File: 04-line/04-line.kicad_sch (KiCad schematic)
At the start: 71 parts, among them J1 Conn_01x10, J2 Conn_01x10, J3 Conn_01x08

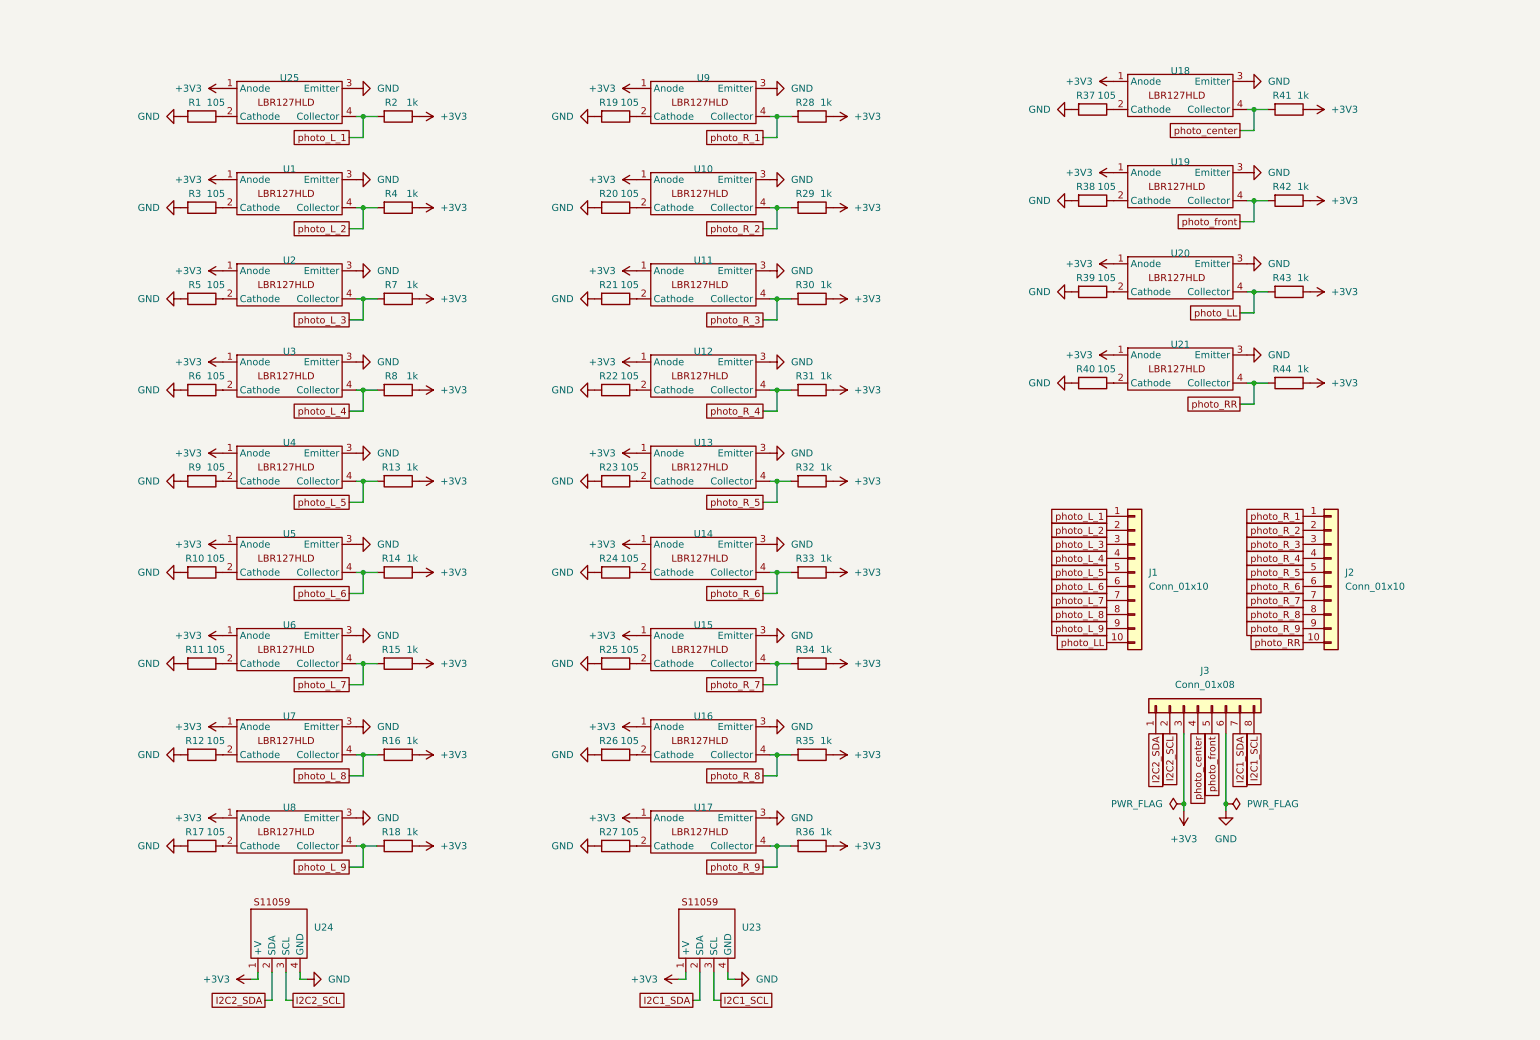
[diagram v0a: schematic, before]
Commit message: がんばる
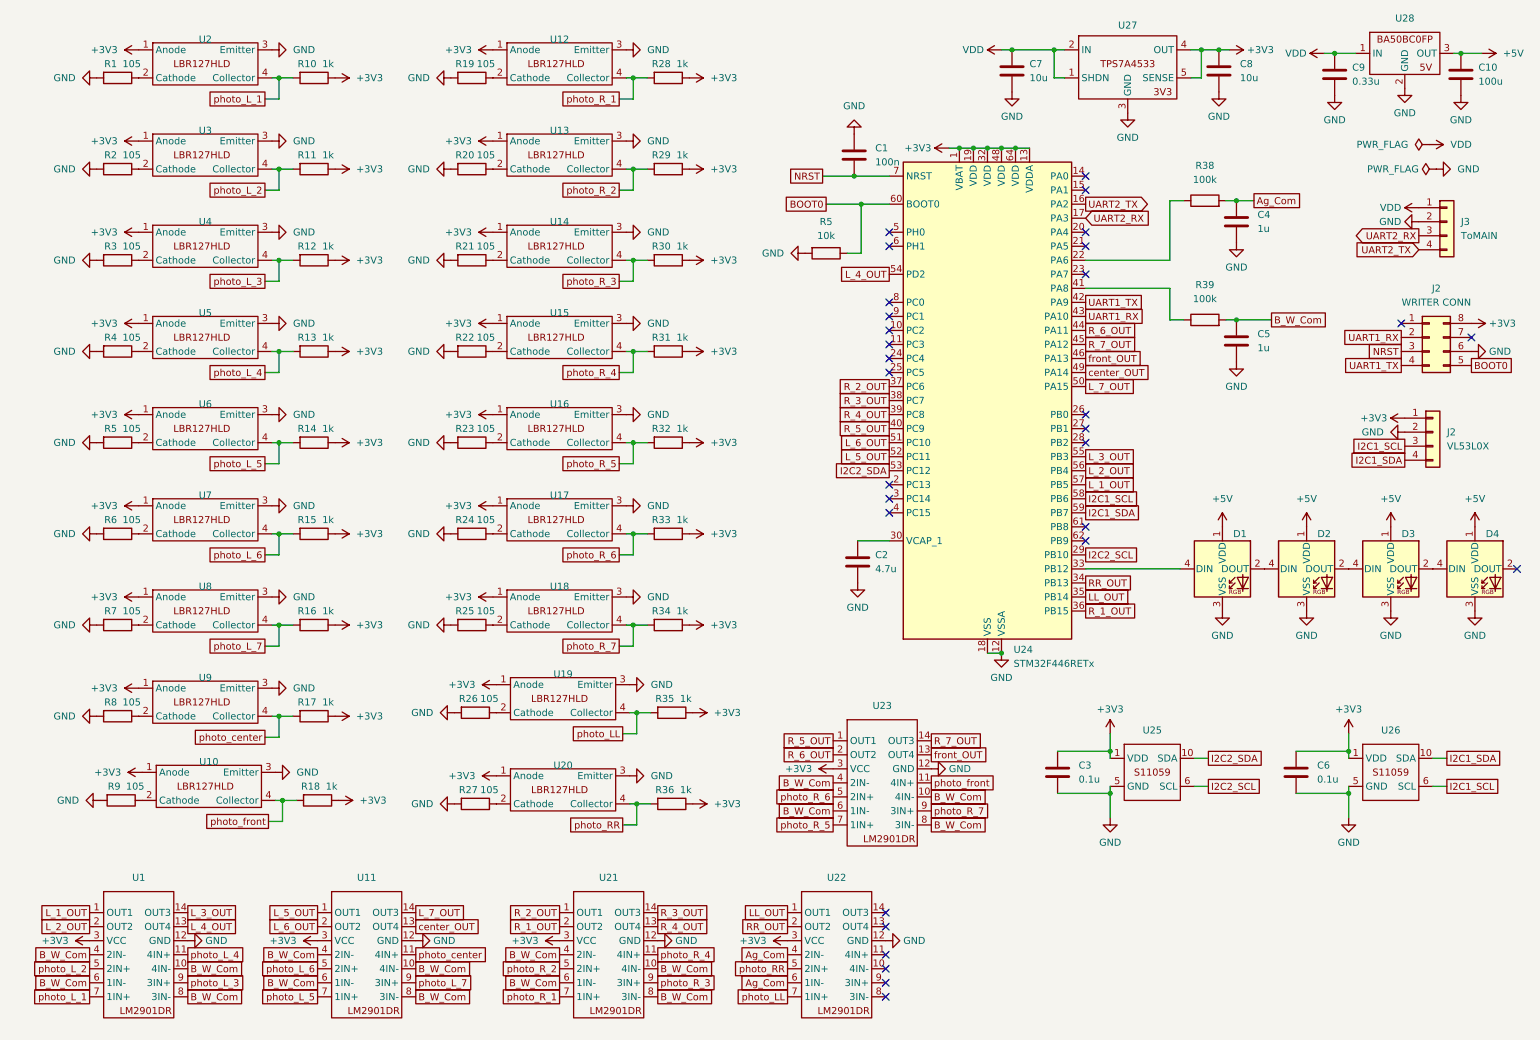
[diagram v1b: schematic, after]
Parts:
- removed J1, J2: Conn_01x10, Connector_PinHeader_2.54mm:PinHeader_1x10_P2.54mm_Vertical, symbol Connector_Generic:Conn_01x10
- removed J3: Conn_01x08, Connector_PinHeader_2.54mm:PinHeader_1x08_P2.54mm_Vertical, symbol Connector_Generic:Conn_01x08
- removed R12, R17, R26, R27: 105, symbol Device:R
- removed R16, R18, R35, R36: 1k, symbol Device:R
- removed U16, U17, U7, U8: ~, symbol akiduki:LBR127HLD
- removed U23, U24: ~, S11059:S11059, symbol S11059:S11059
- added C1: 100n, symbol Device:C
- added C10: 100u, symbol Device:C
- added C2: 4.7u, symbol Device:C
- added C3, C6: 0.1u, symbol Device:C
- added C4, C5: 1u, symbol Device:C
- added C7, C8: 10u, symbol Device:C
- added C9: 0.33u, symbol Device:C
- added D1, D2, D3, D4: WS2812B, LED_SMD:LED_WS2812B_PLCC4_5.0x5.0mm_P3.2mm, symbol LED:WS2812B
- added J2: VL53L0X, Connector_PinHeader_2.54mm:PinHeader_1x04_P2.54mm_Vertical, symbol Connector_Generic:Conn_01x04
- added J2: WRITER CONN, Connector_PinHeader_2.54mm:PinHeader_2x04_P2.54mm_Vertical, symbol Connector_Generic:Conn_02x04_Counter_Clockwise
- added J3: ToMAIN, Connector_JST:JST_XH_B4B-XH-A_1x04_P2.50mm_Vertical, symbol Connector_Generic:Conn_01x04
- added R38, R39: 100k, symbol Device:R
- added R5: 10k, Resistor_SMD:R_0805_2012Metric, symbol Device:R
- added U1, U11, U21, U22, U23: ~, Package_SO:SOIC-14_3.9x8.7mm_P1.27mm, symbol JLCPCB_items:LM2901DR
- added U24: STM32F446RETx, Package_QFP:LQFP-64_10x10mm_P0.5mm, symbol MCU_ST_STM32F4:STM32F446RETx
- added U25, U26: ~, Akiduki:S11059, symbol akiduki:S11059
- added U27: ~, Package_TO_SOT_SMD:SOT-223-6, symbol JLCPCB_items:TPS7A4533DCQR
- added U28: ~, Package_TO_SOT_SMD:TO-252-3_TabPin2, symbol JLCPCB_items:BA50BC0FP
- R1, R19, R20, R21, R22, R23, R24, R25: footprint (none) -> Resistor_SMD:R_0603_1608Metric; LCSC (none) -> C128061
- R10: renamed from R2; footprint (none) -> Resistor_SMD:R_1206_3216Metric; LCSC (none) -> C138242
- R11: renamed from R4; footprint (none) -> Resistor_SMD:R_1206_3216Metric; LCSC (none) -> C138242
- R12: renamed from R7; footprint (none) -> Resistor_SMD:R_1206_3216Metric; LCSC (none) -> C138242
- R13: renamed from R8; footprint (none) -> Resistor_SMD:R_1206_3216Metric; LCSC (none) -> C138242
- R14: renamed from R13; footprint (none) -> Resistor_SMD:R_1206_3216Metric; LCSC (none) -> C138242
- R15: renamed from R14; footprint (none) -> Resistor_SMD:R_1206_3216Metric; LCSC (none) -> C138242
- R16: renamed from R15; footprint (none) -> Resistor_SMD:R_1206_3216Metric; LCSC (none) -> C138242
- R17: renamed from R41; footprint (none) -> Resistor_SMD:R_1206_3216Metric; LCSC (none) -> C138242
- R18: renamed from R42; footprint (none) -> Resistor_SMD:R_1206_3216Metric; LCSC (none) -> C138242
- R2: renamed from R3; footprint (none) -> Resistor_SMD:R_0603_1608Metric; LCSC (none) -> C128061
- R26: renamed from R39; footprint (none) -> Resistor_SMD:R_0603_1608Metric; LCSC (none) -> C128061
- R27: renamed from R40; footprint (none) -> Resistor_SMD:R_0603_1608Metric; LCSC (none) -> C128061
- R28, R29, R30, R31, R32, R33, R34: footprint (none) -> Resistor_SMD:R_1206_3216Metric; LCSC (none) -> C138242
- R3: renamed from R5; footprint (none) -> Resistor_SMD:R_0603_1608Metric; LCSC (none) -> C128061
- R35: renamed from R43; footprint (none) -> Resistor_SMD:R_1206_3216Metric; LCSC (none) -> C138242
- R36: renamed from R44; footprint (none) -> Resistor_SMD:R_1206_3216Metric; LCSC (none) -> C138242
- R4: renamed from R6; footprint (none) -> Resistor_SMD:R_0603_1608Metric; LCSC (none) -> C128061
- R5: renamed from R9; footprint (none) -> Resistor_SMD:R_0603_1608Metric; LCSC (none) -> C128061
- R6: renamed from R10; footprint (none) -> Resistor_SMD:R_0603_1608Metric; LCSC (none) -> C128061
- R7: renamed from R11; footprint (none) -> Resistor_SMD:R_0603_1608Metric; LCSC (none) -> C128061
- R8: renamed from R37; footprint (none) -> Resistor_SMD:R_0603_1608Metric; LCSC (none) -> C128061
- R9: renamed from R38; footprint (none) -> Resistor_SMD:R_0603_1608Metric; LCSC (none) -> C128061
- U10: renamed from U19; footprint (none) -> Akiduki:LBR127HLD
- U12: renamed from U9; footprint (none) -> Akiduki:LBR127HLD
- U13: renamed from U10; footprint (none) -> Akiduki:LBR127HLD
- U14: renamed from U11; footprint (none) -> Akiduki:LBR127HLD
- U15: renamed from U12; footprint (none) -> Akiduki:LBR127HLD
- U16: renamed from U13; footprint (none) -> Akiduki:LBR127HLD
- U17: renamed from U14; footprint (none) -> Akiduki:LBR127HLD
- U18: renamed from U15; footprint (none) -> Akiduki:LBR127HLD
- U19: renamed from U20; footprint (none) -> Akiduki:LBR127HLD
- U2: renamed from U25; footprint (none) -> Akiduki:LBR127HLD
- U20: renamed from U21; footprint (none) -> Akiduki:LBR127HLD
- U3: renamed from U1; footprint (none) -> Akiduki:LBR127HLD
- U4: renamed from U2; footprint (none) -> Akiduki:LBR127HLD
- U5: renamed from U3; footprint (none) -> Akiduki:LBR127HLD
- U6: renamed from U4; footprint (none) -> Akiduki:LBR127HLD
- U7: renamed from U5; footprint (none) -> Akiduki:LBR127HLD
- U8: renamed from U6; footprint (none) -> Akiduki:LBR127HLD
- U9: renamed from U18; footprint (none) -> Akiduki:LBR127HLD
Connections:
- net +3V3: now also C3.1, C6.1, C8.1, J2.1 (Pin_1), J2.8 (Pin_8), U1.3 (VCC), U11.3 (VCC), U21.3 (VCC), U22.3 (VCC), U23.3 (VCC), U24.1 (VBAT), U24.13 (VDDA), U24.19 (VDD), U24.32 (VDD), U24.48 (VDD), U24.64 (VDD), U25.1 (VDD), U26.1 (VDD), U27.4 (OUT), U27.5 (SENSE)
- net GND: now also C1.1, C10.2, C2.2, C3.2, C4.2, C5.2, C6.2, C7.2, C8.2, C9.2, D1.3 (VSS), D2.3 (VSS), D3.3 (VSS), D4.3 (VSS), J2.2 (Pin_2), J2.6 (Pin_6), J3.2 (Pin_2), R5.2, U1.12 (GND), U11.12 (GND), U21.12 (GND), U22.12 (GND), U23.12 (GND), U24.12 (VSSA), U24.18 (VSS), U24.31 (VSS), U24.47 (VSS), U24.63 (VSS), U25.5 (GND), U26.5 (GND), U27.3 (GND), U27.6 (GND), U28.2 (GND)
- net I2C1_SCL: now also J2.3 (Pin_3), U24.58 (PB6), U26.6 (SCL)
- net I2C1_SDA: now also J2.4 (Pin_4), U24.59 (PB7), U26.10 (SDA)
- net I2C2_SCL: now also U24.29 (PB10), U25.6 (SCL)
- net I2C2_SDA: now also U24.53 (PC12), U25.10 (SDA)
- net photo_LL: now also U22.7 (1IN+)
- net photo_L_1: now also U1.7 (1IN+)
- net photo_L_2: now also U1.5 (2IN+)
- net photo_L_3: now also U1.9 (3IN+)
- net photo_L_4: now also U1.11 (4IN+)
- net photo_L_5: now also U11.7 (1IN+)
- net photo_L_6: now also U11.5 (2IN+)
- net photo_L_7: now also U11.9 (3IN+)
- net photo_RR: now also U22.5 (2IN+)
- net photo_R_1: now also U21.7 (1IN+)
- net photo_R_2: now also U21.5 (2IN+)
- net photo_R_3: now also U21.9 (3IN+)
- net photo_R_4: now also U21.11 (4IN+)
- net photo_R_5: now also U23.7 (1IN+)
- net photo_R_6: now also U23.5 (2IN+)
- net photo_R_7: now also U23.9 (3IN+)
- net photo_center: now also U11.11 (4IN+)
- net photo_front: now also U23.11 (4IN+)
- new net: D2.2 (DOUT), D3.4 (DIN)
- new net: D1.2 (DOUT), D2.4 (DIN)
- new net: D1.4 (DIN), U24.33 (PB12)
- new net: R39.1, U24.41 (PA8)
- new net: R38.1, U24.22 (PA6)
- new net: C2.1, U24.30 (VCAP_1)
- new net: D3.2 (DOUT), D4.4 (DIN)
- new net +5V: C10.1, D1.1 (VDD), D2.1 (VDD), D3.1 (VDD), D4.1 (VDD), U28.3 (OUT)
- new net Ag_Com: C4.1, R38.2, U22.4 (2IN-), U22.6 (1IN-)
- new net BOOT0: J2.5 (Pin_5), R5.1, U24.60 (BOOT0)
- new net B_W_Com: C5.1, R39.2, U1.10 (4IN-), U1.4 (2IN-), U1.6 (1IN-), U1.8 (3IN-), U11.10 (4IN-), U11.4 (2IN-), U11.6 (1IN-), U11.8 (3IN-), U21.10 (4IN-), U21.4 (2IN-), U21.6 (1IN-), U21.8 (3IN-), U23.10 (4IN-), U23.4 (2IN-), U23.6 (1IN-), U23.8 (3IN-)
- new net LL_OUT: U22.1 (OUT1), U24.35 (PB14)
- new net L_1_OUT: U1.1 (OUT1), U24.57 (PB5)
- new net L_2_OUT: U1.2 (OUT2), U24.56 (PB4)
- new net L_3_OUT: U1.14 (OUT3), U24.55 (PB3)
- new net L_4_OUT: U1.13 (OUT4), U24.54 (PD2)
- new net L_5_OUT: U11.1 (OUT1), U24.52 (PC11)
- new net L_6_OUT: U11.2 (OUT2), U24.51 (PC10)
- new net L_7_OUT: U11.14 (OUT3), U24.50 (PA15)
- new net NRST: C1.2, J2.3 (Pin_3), U24.7 (NRST)
- new net RR_OUT: U22.2 (OUT2), U24.34 (PB13)
- new net R_1_OUT: U21.2 (OUT2), U24.36 (PB15)
- new net R_2_OUT: U21.1 (OUT1), U24.37 (PC6)
- new net R_3_OUT: U21.14 (OUT3), U24.38 (PC7)
- new net R_4_OUT: U21.13 (OUT4), U24.39 (PC8)
- new net R_5_OUT: U23.1 (OUT1), U24.40 (PC9)
- new net R_6_OUT: U23.2 (OUT2), U24.44 (PA11)
- new net R_7_OUT: U23.14 (OUT3), U24.45 (PA12)
- new net UART1_RX: J2.2 (Pin_2), U24.43 (PA10)
- new net UART1_TX: J2.4 (Pin_4), U24.42 (PA9)
- new net UART2_RX: J3.3 (Pin_3), U24.17 (PA3)
- new net UART2_TX: J3.4 (Pin_4), U24.16 (PA2)
- new net VDD: C7.1, C9.1, J3.1 (Pin_1), U27.1 (SHDN), U27.2 (IN), U28.1 (IN)
- new net center_OUT: U11.13 (OUT4), U24.49 (PA14)
- new net front_OUT: U23.13 (OUT4), U24.46 (PA13)
- no-connect marks 0 -> 30
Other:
- title: (none) -> 04-LINE
- moved on the sheet: R1, R10, R11, R12, R13, R14, R15, R16, R17, R18, R19, R2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

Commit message: line...
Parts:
- C1, C10, C2, C3, C4, C5, C6, C7, C8, C9: footprint (none) -> Capacitor_SMD:C_0805_2012Metric
- R38, R39: footprint (none) -> Resistor_SMD:R_0805_2012Metric
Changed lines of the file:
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@@
       (effects (font (size 1.27 1.27)) (justify left))
     )
-    (property "Footprint" "" (at 200.3552 154.305 0)
+    (property "Footprint" "Capacitor_SMD:C_0805_2012Metric" (at 200.3552 154.305 0)
       (effects (font (size 1.27 1.27)) hide)
     )
@@
       (effects (font (size 1.27 1.27)) (justify left))
     )
-    (property "Footprint" "" (at 229.5652 27.305 0)
+    (property "Footprint" "Capacitor_SMD:C_0805_2012Metric" (at 229.5652 27.305 0)
       (effects (font (size 1.27 1.27)) hide)
     )
@@
       (effects (font (size 1.27 1.27)) (justify left))
     )
-    (property "Footprint" "" (at 163.5252 42.545 0)
+    (property "Footprint" "Capacitor_SMD:C_0805_2012Metric" (at 163.5252 42.545 0)
       (effects (font (size 1.27 1.27)) hide)
     )
@@
       (effects (font (size 1.27 1.27)) (justify left))
     )
-    (property "Footprint" "" (at 192.1002 27.305 0)
+    (property "Footprint" "Capacitor_SMD:C_0805_2012Metric" (at 192.1002 27.305 0)
       (effects (font (size 1.27 1.27)) hide)
     )
@@
       (effects (font (size 1.27 1.27)) (justify left))
     )
-    (property "Footprint" "" (at 232.7402 54.61 0)
+    (property "Footprint" "Capacitor_SMD:C_0805_2012Metric" (at 232.7402 54.61 0)
       (effects (font (size 1.27 1.27)) hide)
     )
@@
       (effects (font (size 1.27 1.27)) (justify left))
     )
-    (property "Footprint" "" (at 273.3802 27.94 0)
+    (property "Footprint" "Capacitor_SMD:C_0805_2012Metric" (at 273.3802 27.94 0)
       (effects (font (size 1.27 1.27)) hide)
     )
@@
       (effects (font (size 1.27 1.27)) (justify left))
     )
-    (property "Footprint" "" (at 250.5202 27.94 0)
+    (property "Footprint" "Capacitor_SMD:C_0805_2012Metric" (at 250.5202 27.94 0)
       (effects (font (size 1.27 1.27)) hide)
     )
@@
       (effects (font (size 1.27 1.27)))
     )
-    (property "Footprint" "" (at 226.06 70.358 90)
+    (property "Footprint" "Resistor_SMD:R_0805_2012Metric" (at 226.06 70.358 90)
       (effects (font (size 1.27 1.27)) hide)
     )
@@
       (effects (font (size 1.27 1.27)))
     )
-    (property "Footprint" "" (at 226.06 48.768 90)
+    (property "Footprint" "Resistor_SMD:R_0805_2012Metric" (at 226.06 48.768 90)
       (effects (font (size 1.27 1.27)) hide)
     )
@@
       (effects (font (size 1.27 1.27)) (justify left))
     )
-    (property "Footprint" "" (at 232.7402 76.2 0)
+    (property "Footprint" "Capacitor_SMD:C_0805_2012Metric" (at 232.7402 76.2 0)
       (effects (font (size 1.27 1.27)) hide)
     )
@@
       (effects (font (size 1.27 1.27)) (justify left))
     )
-    (property "Footprint" "" (at 243.5352 154.305 0)
+    (property "Footprint" "Capacitor_SMD:C_0805_2012Metric" (at 243.5352 154.305 0)
       (effects (font (size 1.27 1.27)) hide)
     )
@@
       (effects (font (size 1.27 1.27)) (justify left))
     )
-    (property "Footprint" "" (at 164.1602 116.205 0)
+    (property "Footprint" "Capacitor_SMD:C_0805_2012Metric" (at 164.1602 116.205 0)
       (effects (font (size 1.27 1.27)) hide)
     )
